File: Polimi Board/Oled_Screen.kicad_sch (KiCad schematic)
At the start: 1 part, among them J5 Conn_01x04_Socket

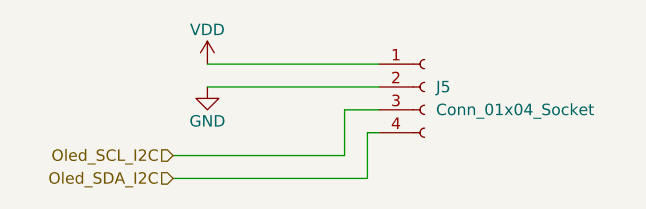
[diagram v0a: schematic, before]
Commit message: Finish schematic part
To be reviewd
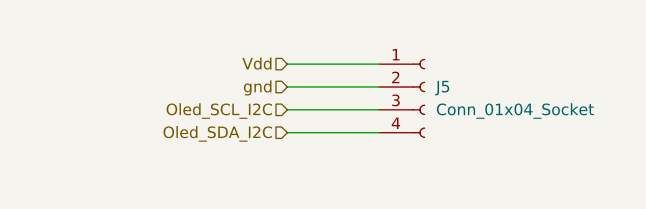
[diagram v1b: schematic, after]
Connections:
- net GND renamed gnd
- net VDD renamed Vdd
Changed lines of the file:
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@@
   (title_block
     (title "Polimi Board ")
-    (date "2024-04-09")
+    (date "2024-04-24")
     (rev "1.0")
     (company "Politecnico di Milano")
-    (comment 1 "Embedded Systems")
+    (comment 1 "Embedded Systems Project")
     (comment 2 "ing. Zaccaria Eliseo Carrettoni")
   )
-  (wire (pts (xy 129.54 96.52) (xy 130.81 96.52))
+  (wire (pts (xy 120.65 96.52) (xy 130.81 96.52))
     (stroke (width 0) (type default))
   )
-  (wire (pts (xy 127 93.98) (xy 127 99.06))
+  (wire (pts (xy 120.65 91.44) (xy 130.81 91.44))
     (stroke (width 0) (type default))
   )
-  (wire (pts (xy 111.76 91.44) (xy 130.81 91.44))
+  (wire (pts (xy 120.65 88.9) (xy 130.81 88.9))
     (stroke (width 0) (type default))
   )
-  (wire (pts (xy 107.95 101.6) (xy 129.54 101.6))
+  (wire (pts (xy 120.65 93.98) (xy 130.81 93.98))
     (stroke (width 0) (type default))
   )
-  (wire (pts (xy 111.76 88.9) (xy 130.81 88.9))
-    (stroke (width 0) (type default))
-  )
-  (wire (pts (xy 107.95 99.06) (xy 127 99.06))
-    (stroke (width 0) (type default))
-  )
-  (wire (pts (xy 129.54 96.52) (xy 129.54 101.6))
-    (stroke (width 0) (type default))
-  )
-  (wire (pts (xy 127 93.98) (xy 130.81 93.98))
-    (stroke (width 0) (type default))
-  )
-  (hierarchical_label "Oled_SDA_I2C" (shape input) (at 107.95 101.6 180) (fields_autoplaced)
+  (hierarchical_label "Oled_SDA_I2C" (shape input) (at 120.65 96.52 180) (fields_autoplaced)
     (effects (font (size 1.27 1.27)) (justify right))
   )
-  (hierarchical_label "Oled_SCL_I2C" (shape input) (at 107.95 99.06 180) (fields_autoplaced)
+  (hierarchical_label "Oled_SCL_I2C" (shape input) (at 120.65 93.98 180) (fields_autoplaced)
     (effects (font (size 1.27 1.27)) (justify right))
   )
-  (symbol (lib_id "power:VDD") (at 111.76 88.9 0) (unit 1)
-    (in_bom yes) (on_board yes) (dnp no)
-    (property "Reference" "#PWR026" (at 111.76 92.71 0)
-      (effects (font (size 1.27 1.27)) hide)
-    )
-    (property "Value" "VDD" (at 111.76 85.09 0)
-      (effects (font (size 1.27 1.27)))
-    )
-    (property "Footprint" "" (at 111.76 88.9 0)
-      (effects (font (size 1.27 1.27)) hide)
-    )
-    (property "Datasheet" "" (at 111.76 88.9 0)
-      (effects (font (size 1.27 1.27)) hide)
-    )
-    (pin "1")
-    (instances
-      (project "Polimi Board"
-        (path "/319fe76e-1f98-44b3-99b0-af1a9ad7322c/108d9b54-87bf-4732-a1b8-edcdb25241bc"
-          (reference "#PWR026") (unit 1)
-        )
-      )
-    )
+  (hierarchical_label "gnd" (shape input) (at 120.65 91.44 180) (fields_autoplaced)
+    (effects (font (size 1.27 1.27)) (justify right))
+  )
+  (hierarchical_label "Vdd" (shape input) (at 120.65 88.9 180) (fields_autoplaced)
+    (effects (font (size 1.27 1.27)) (justify right))
   )
   (symbol (lib_id "Connector:Conn_01x04_Socket") (at 135.89 91.44 0) (unit 1)
@@
         )
       )
-    )
-  )
-  (symbol (lib_id "power:GND") (at 111.76 91.44 0) (unit 1)
-    (in_bom yes) (on_board yes) (dnp no)
-    (property "Reference" "#PWR027" (at 111.76 97.79 0)
-      (effects (font (size 1.27 1.27)) hide)
-    )
-    (property "Value" "GND" (at 111.76 95.25 0)
-      (effects (font (size 1.27 1.27)))
-    )
-    (property "Footprint" "" (at 111.76 91.44 0)
-      (effects (font (size 1.27 1.27)) hide)
-    )
-    (property "Datasheet" "" (at 111.76 91.44 0)
-      (effects (font (size 1.27 1.27)) hide)
-    )
-    (pin "1")
-    (instances
-      (project "Polimi Board"
-        (path "/319fe76e-1f98-44b3-99b0-af1a9ad7322c/108d9b54-87bf-4732-a1b8-edcdb25241bc"
-          (reference "#PWR027") (unit 1)
-        )
-      )
